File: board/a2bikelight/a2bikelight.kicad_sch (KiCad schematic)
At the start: 29 parts, among them J1 Barrel_Jack_Switch, J2 Conn_01x02_Male, J3 Conn_01x04_Male, J4 Conn_01x06_Male, J5 Conn_01x02_Male, J6 Conn_01x08_Male, Q1 Si2301CDS, SW1 SW_Push, SW2 SW_Push, U1 STM8L151K4U, U2 AMS1117-3.3, U3 MXC6655XA

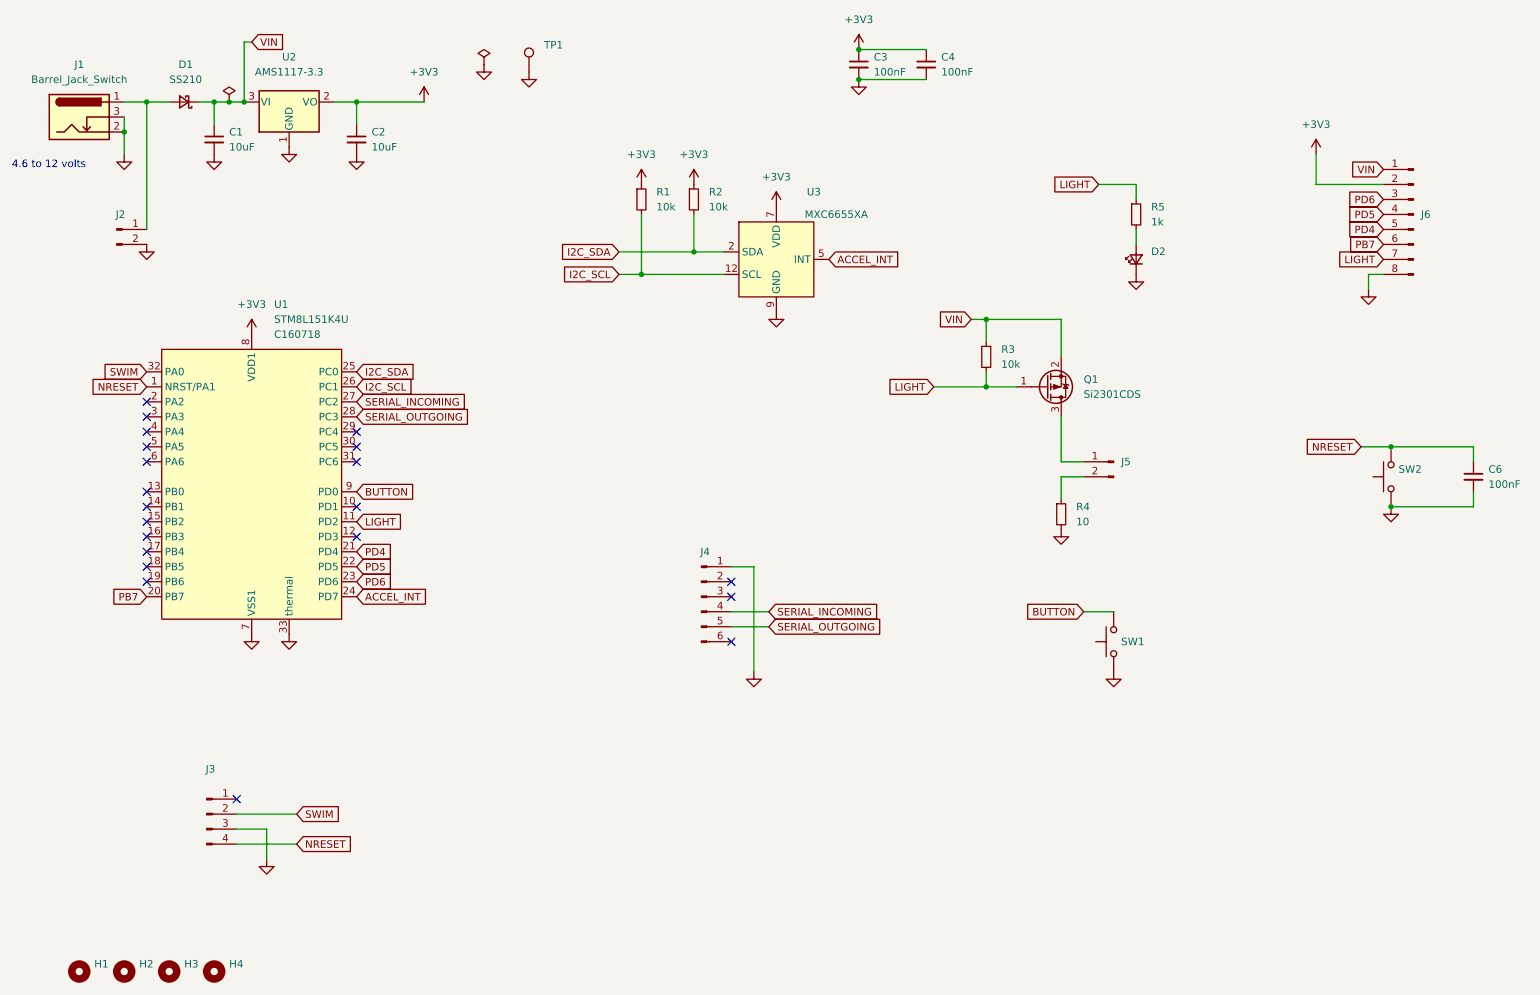
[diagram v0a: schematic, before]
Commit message: kicad 7; fabrication outputs
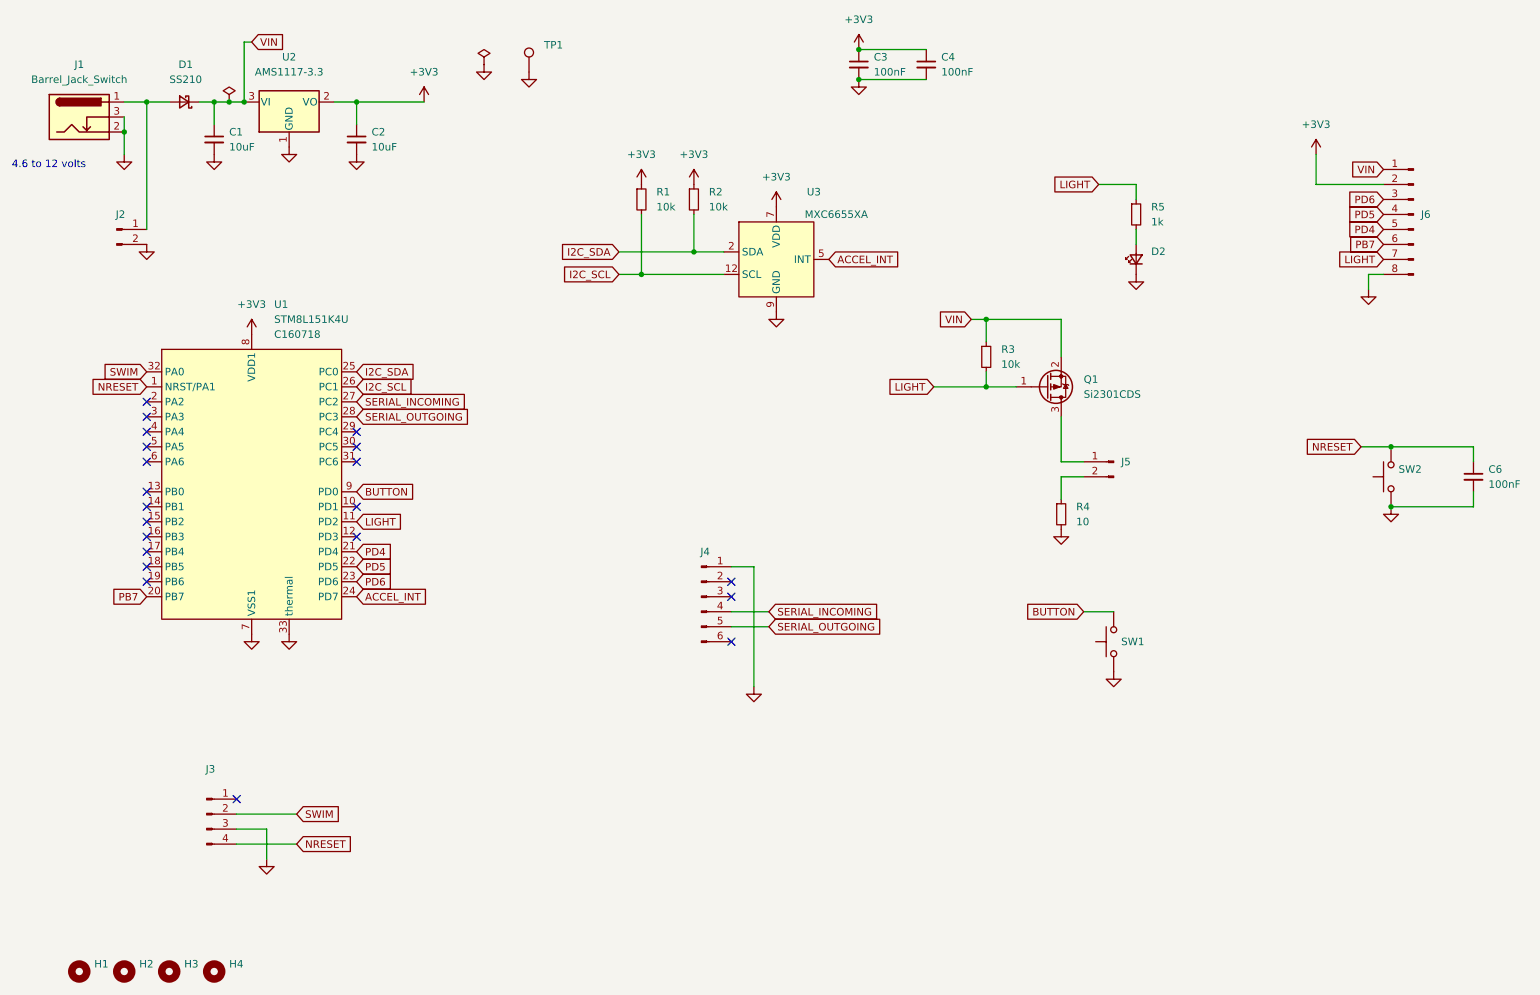
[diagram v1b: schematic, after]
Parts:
- J1, J2, SW1, SW2, U3: now left out of the parts list
